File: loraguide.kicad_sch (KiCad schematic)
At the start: 19 parts, among them J1 USB_C_Receptacle_USB2.0_14P, J2 Conn_Coaxial, SW1 RST, SW2 BOOT, U1 ESP32-S3-WROOM-1, U2 SX1262IMLTRT, U3 AMS1117-3.3

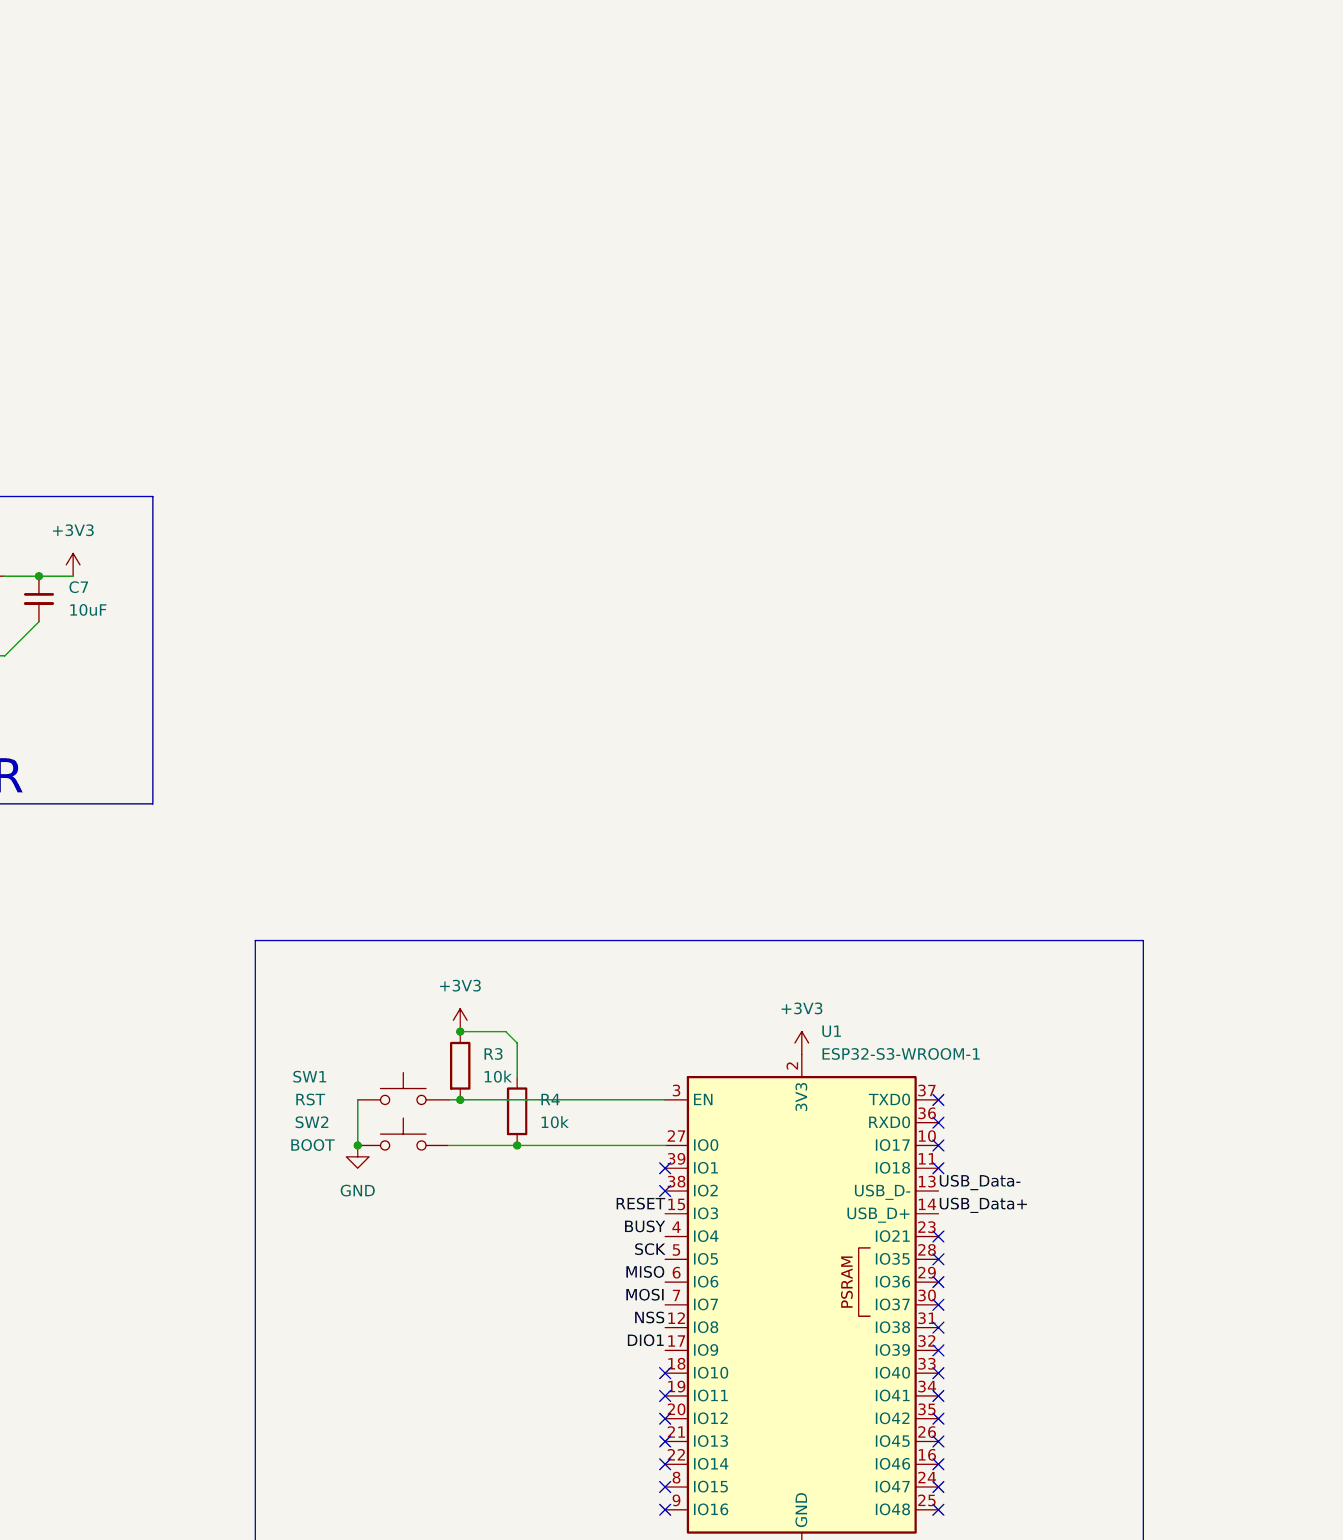
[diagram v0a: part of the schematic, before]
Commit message: upload
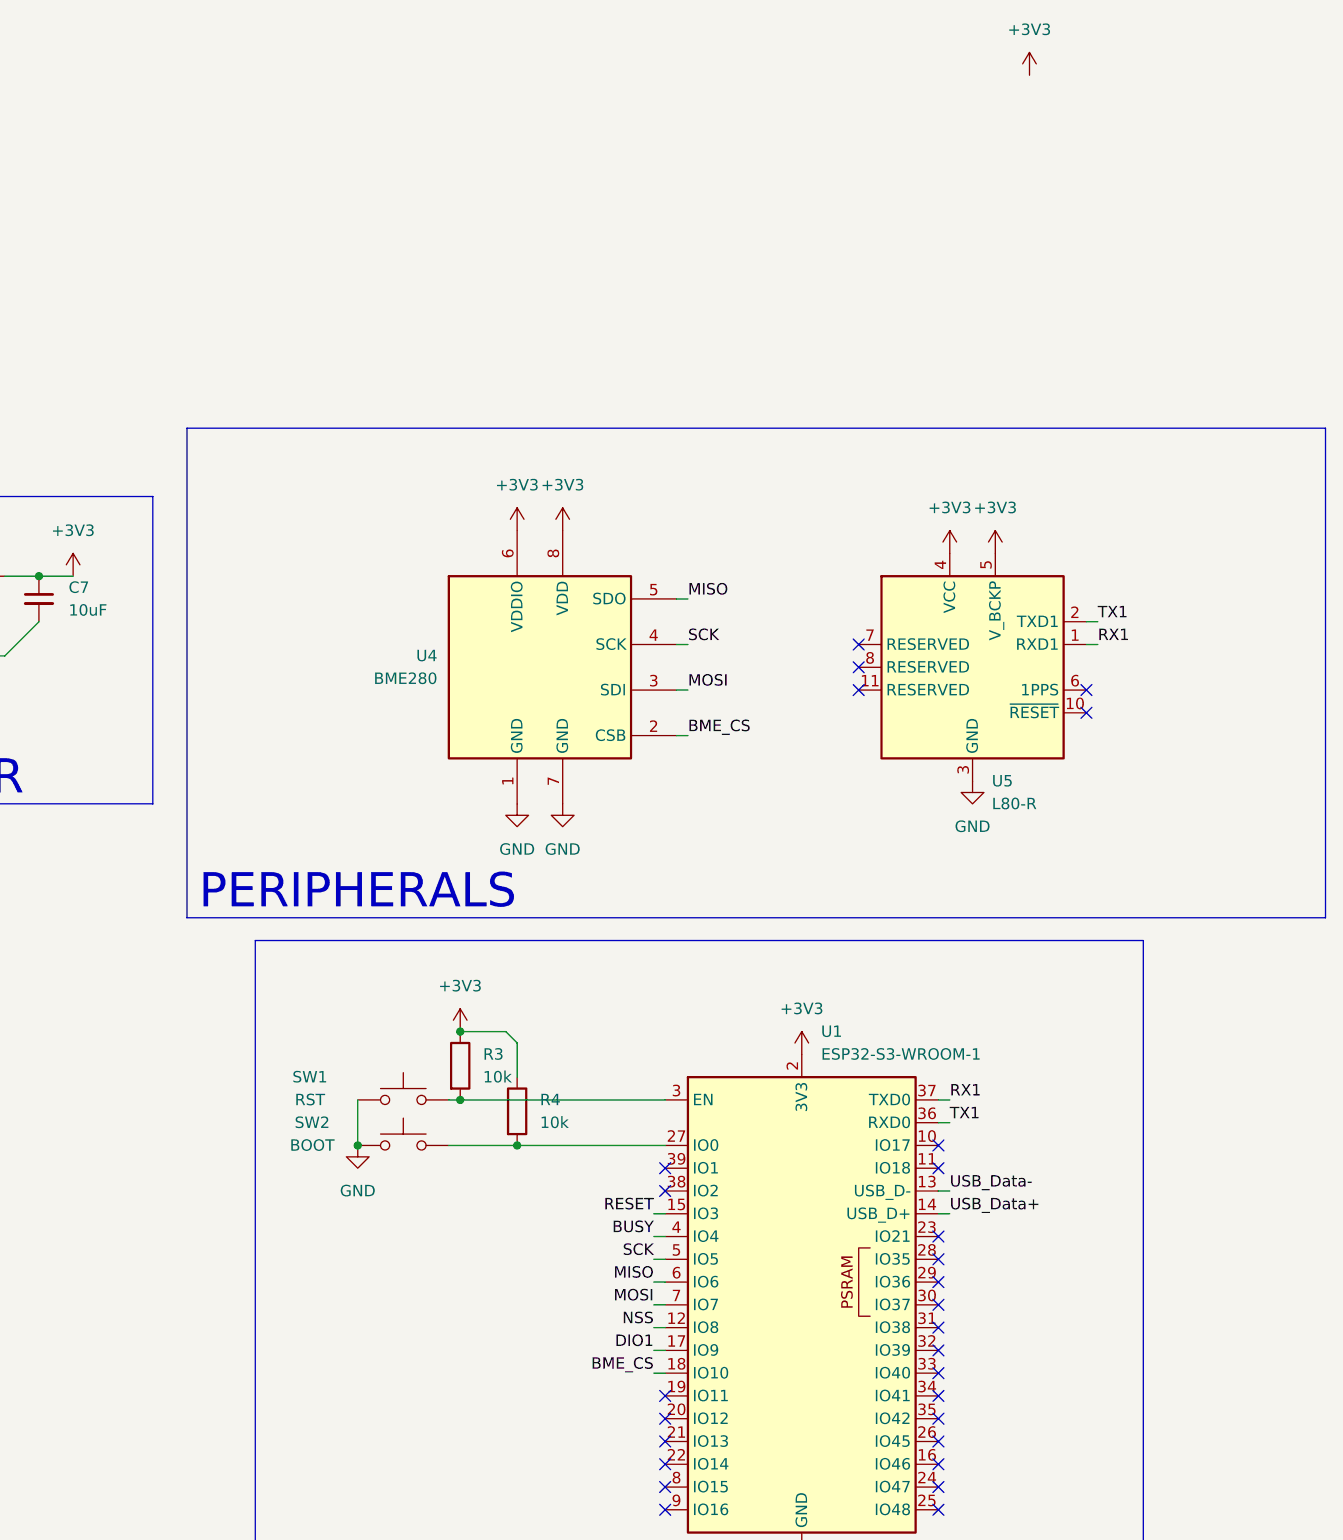
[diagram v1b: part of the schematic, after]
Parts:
- added U4: BME280, Package_LGA:Bosch_LGA-8_2.5x2.5mm_P0.65mm_ClockwisePinNumbering, symbol Sensor:BME280
- added U5: L80-R, RF_GPS:Quectel_L80-R, symbol RF_GPS:L80-R
- L1: footprint Inductor_SMD:L_0402_1005Metric -> Inductor_SMD:L_0603_1608Metric
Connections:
- net +3V3: now also U4.6 (VDDIO), U4.8 (VDD), U5.4 (VCC), U5.5 (V_BCKP)
- net GND: now also U4.1 (GND), U4.7 (GND), U5.12 (GND), U5.3 (GND)
- net MISO: now also U4.5 (SDO)
- net MOSI: now also U4.3 (SDI)
- net SCK: now also U4.4 (SCK)
- net BME_CS: now reaches U1.18 (IO10)
- net BME_CS: now also U4.2 (CSB)
- net TX1: now reaches U1.36 (RXD0)
- net TX1: now also U5.2 (TXD1)
- net RX1: now reaches U1.37 (TXD0)
- net RX1: now also U5.1 (RXD1)
- no-connect marks 32 -> 34
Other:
- note added: "PERIPHERALS"
